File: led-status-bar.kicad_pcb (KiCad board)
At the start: 2 copper layers, 19.3 x 37.2 mm, 21 parts, among them J1 Conn_01x04, J2 Conn_01x04, Q1 2N7002, Q2 2N7002

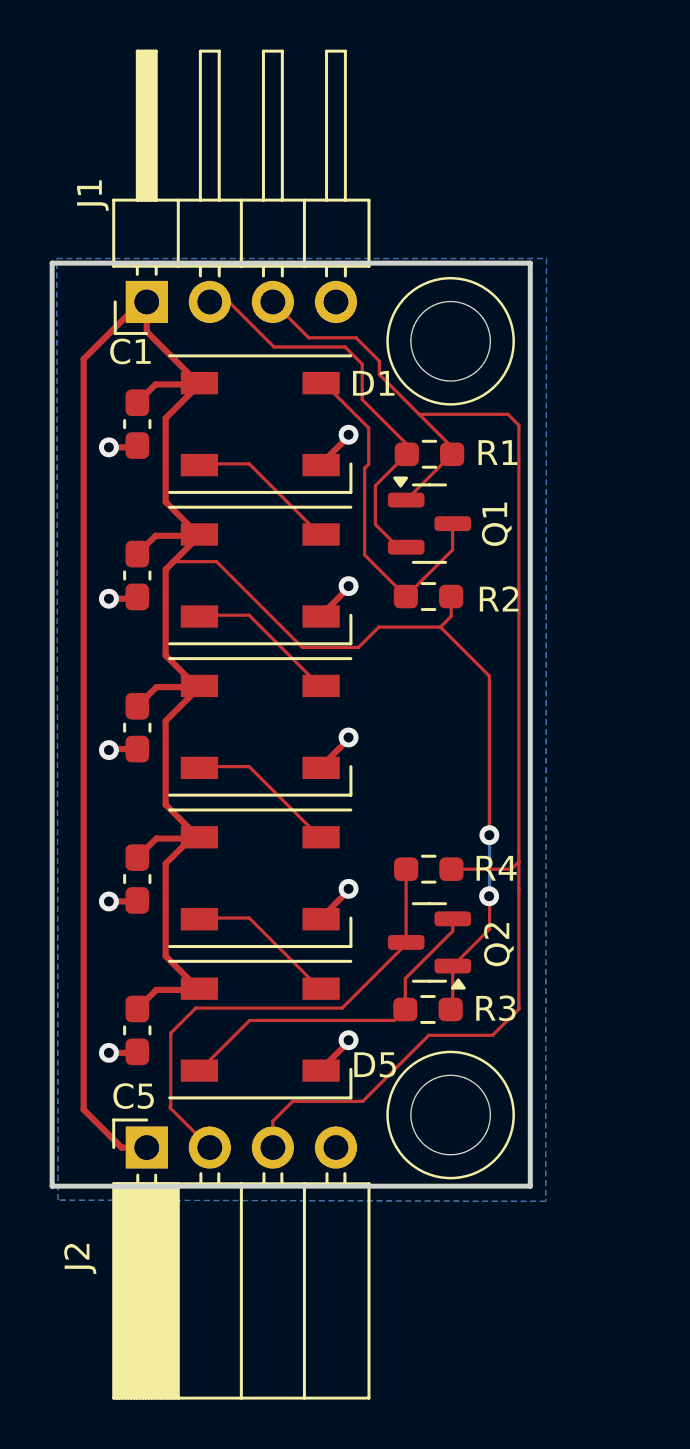
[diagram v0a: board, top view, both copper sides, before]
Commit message: Changes of uids - done by KiCad
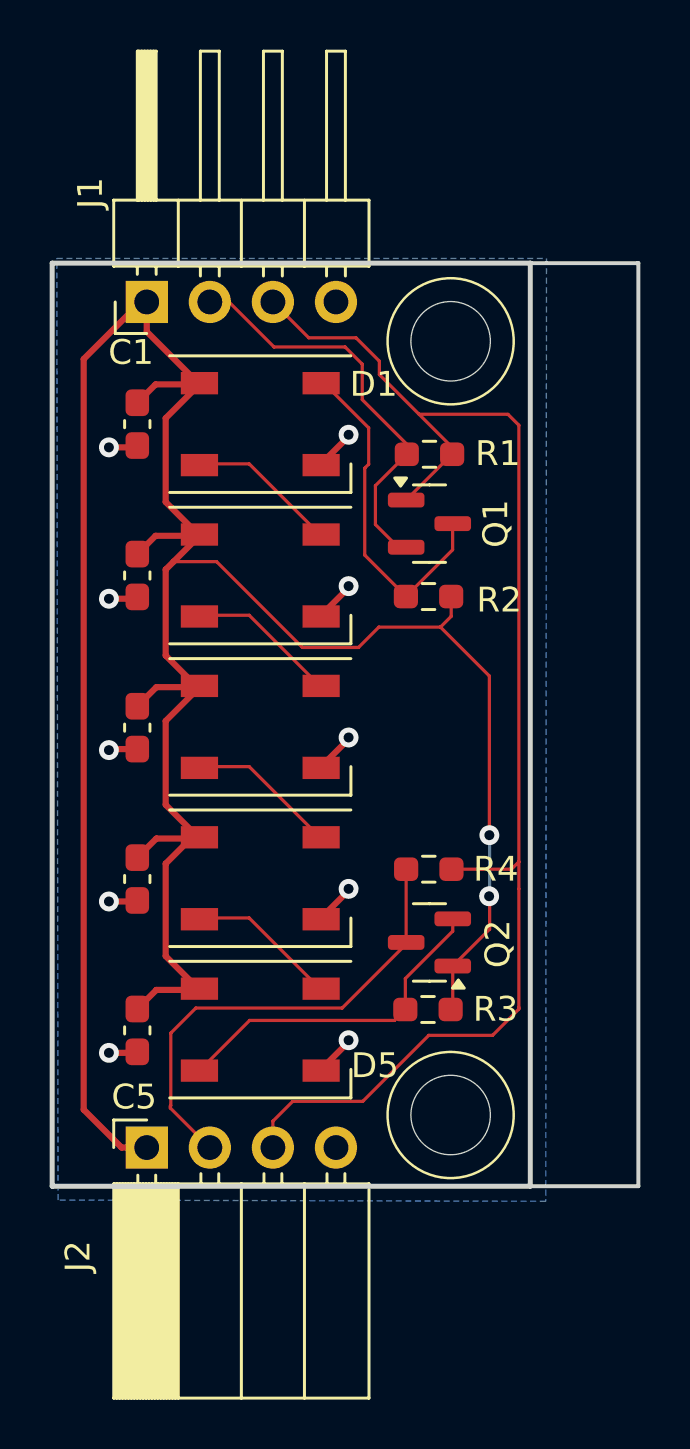
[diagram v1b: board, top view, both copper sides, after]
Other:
- board size 19.3 x 37.2 mm -> 23.6 x 37.2 mm
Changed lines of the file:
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@@
 			(pintype "input")
 		)
-		(model "${KICAD8_3DMODEL_DIR}/LED_SMD.3dshapes/LED_WS2812B_PLCC4_5.0x5.0mm_P3.2mm.wrl"
+		(model "${KISYS3DMOD}/LED_SMD.3dshapes/LED_WS2812B_PLCC4_5.0x5.0mm_P3.2mm.step"
 			(offset
 				(xyz 0 0 0)
@@
 			(pintype "input")
 		)
-		(model "${KICAD8_3DMODEL_DIR}/LED_SMD.3dshapes/LED_WS2812B_PLCC4_5.0x5.0mm_P3.2mm.wrl"
+		(model "${KISYS3DMOD}/LED_SMD.3dshapes/LED_WS2812B_PLCC4_5.0x5.0mm_P3.2mm.step"
 			(offset
 				(xyz 0 0 0)
@@
 			(pintype "input")
 		)
-		(model "${KICAD8_3DMODEL_DIR}/LED_SMD.3dshapes/LED_WS2812B_PLCC4_5.0x5.0mm_P3.2mm.wrl"
+		(model "${KISYS3DMOD}/LED_SMD.3dshapes/LED_WS2812B_PLCC4_5.0x5.0mm_P3.2mm.step"
 			(offset
 				(xyz 0 0 0)
@@
 			(pintype "input")
 		)
-		(model "${KICAD8_3DMODEL_DIR}/LED_SMD.3dshapes/LED_WS2812B_PLCC4_5.0x5.0mm_P3.2mm.wrl"
+		(model "${KISYS3DMOD}/LED_SMD.3dshapes/LED_WS2812B_PLCC4_5.0x5.0mm_P3.2mm.step"
 			(offset
 				(xyz 0 0 0)
@@
 			(pintype "input")
 		)
-		(model "${KICAD8_3DMODEL_DIR}/LED_SMD.3dshapes/LED_WS2812B_PLCC4_5.0x5.0mm_P3.2mm.wrl"
+		(model "${KISYS3DMOD}/LED_SMD.3dshapes/LED_WS2812B_PLCC4_5.0x5.0mm_P3.2mm.step"
 			(offset
 				(xyz 0 0 0)
@@
 		)
 	)
+  (gr_line (start 122.682000 73.352000) (end 146.289749 73.352000) (layer Edge.Cuts) (width 0.16))
+  (gr_line (start 146.289749 73.352000) (end 146.289749 110.526000) (layer Edge.Cuts) (width 0.16))
+  (gr_line (start 146.289749 110.526000) (end 122.682000 110.526000) (layer Edge.Cuts) (width 0.16))
+  (gr_line (start 122.682000 110.526000) (end 122.682000 73.352000) (layer Edge.Cuts) (width 0.16))
 )
